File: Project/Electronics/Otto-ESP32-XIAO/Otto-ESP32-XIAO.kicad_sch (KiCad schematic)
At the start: 29 parts, among them J1 Conn_01x03, J10 Conn_01x02, J11 Conn_01x04, J12 OLED 0,91" - I2C (SKU21796), J2 Conn_01x03, J3 Conn_01x03, J4 Conn_01x03, J5 Conn_01x03, J6 Conn_01x03, J7 Conn_01x04, J8 Conn_01x06, J9 Conn_01x04, SW1 SW_SPDT, U1 MOUDLE-SEEEDUINO-XIAO-ESP32C3, U2 R-78E5.0-1.0, U3 TMC2208_SILENTSTEPSTICK, U4 TMC2208_SILENTSTEPSTICK

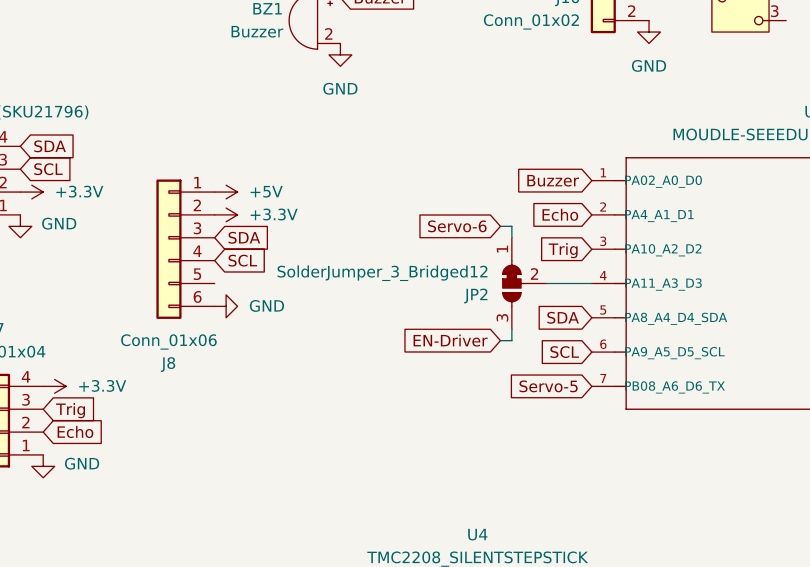
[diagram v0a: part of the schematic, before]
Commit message: quick update
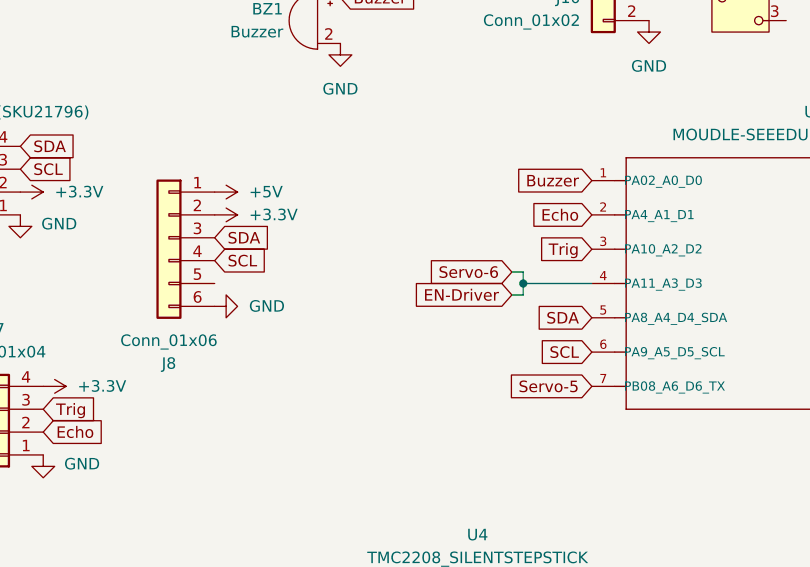
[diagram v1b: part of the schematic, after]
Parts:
- removed JP2: SolderJumper_3_Bridged12, Jumper:SolderJumper-3_P1.3mm_Bridged12_RoundedPad1.0x1.5mm, symbol Jumper:SolderJumper_3_Bridged12
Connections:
- net Servo-6 is gone; now on net EN-Driver: J6.1 (Pin_1)
- net EN-Driver: now also U1.4 (PA11_A3_D3)
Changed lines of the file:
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@@
 	)
 	(junction
+		(at 114.3 88.9)
+		(diameter 0)
+		(color 0 0 0 0)
+	)
+	(junction
 		(at 200.66 102.87)
 		(diameter 0)
@@
 	(wire
 		(pts
-			(xy 113.03 95.25) (xy 113.03 93.98)
+			(xy 213.36 102.87) (xy 200.66 102.87)
 		)
 		(stroke
@@
 	(wire
 		(pts
-			(xy 213.36 102.87) (xy 200.66 102.87)
+			(xy 213.36 111.76) (xy 200.66 111.76)
 		)
 		(stroke
@@
 	(wire
 		(pts
-			(xy 213.36 111.76) (xy 200.66 111.76)
+			(xy 114.3 88.9) (xy 121.92 88.9)
 		)
 		(stroke
@@
 	(wire
 		(pts
-			(xy 111.76 82.55) (xy 113.03 82.55)
+			(xy 194.31 144.78) (xy 191.77 144.78)
 		)
 		(stroke
@@
 	(wire
 		(pts
-			(xy 194.31 144.78) (xy 191.77 144.78)
+			(xy 114.3 87.63) (xy 114.3 88.9)
 		)
 		(stroke
@@
 	(wire
 		(pts
-			(xy 200.66 102.87) (xy 200.66 100.33)
+			(xy 113.03 90.17) (xy 114.3 90.17)
 		)
 		(stroke
@@
 	(wire
 		(pts
-			(xy 127 139.7) (xy 129.54 137.16)
+			(xy 200.66 102.87) (xy 200.66 100.33)
 		)
 		(stroke
@@
 	(wire
 		(pts
-			(xy 127 137.16) (xy 129.54 139.7)
+			(xy 113.03 87.63) (xy 114.3 87.63)
 		)
 		(stroke
@@
 	(wire
 		(pts
-			(xy 116.84 88.9) (xy 121.92 88.9)
+			(xy 127 139.7) (xy 129.54 137.16)
 		)
 		(stroke
@@
 	(wire
 		(pts
-			(xy 111.76 95.25) (xy 113.03 95.25)
+			(xy 127 137.16) (xy 129.54 139.7)
 		)
 		(stroke
@@
 	(wire
 		(pts
-			(xy 200.66 111.76) (xy 200.66 102.87)
+			(xy 114.3 88.9) (xy 114.3 90.17)
 		)
 		(stroke
@@
 	(wire
 		(pts
-			(xy 191.77 137.16) (xy 194.31 139.7)
+			(xy 200.66 111.76) (xy 200.66 102.87)
 		)
 		(stroke
@@
 	(wire
 		(pts
-			(xy 113.03 82.55) (xy 113.03 83.82)
+			(xy 191.77 137.16) (xy 194.31 139.7)
 		)
 		(stroke
@@
 	(global_label "Servo-6"
 		(shape input)
-		(at 111.76 82.55 180)
+		(at 113.03 87.63 180)
 		(fields_autoplaced yes)
 		(effects
@@
 		)
 		(property "Intersheetrefs" "${INTERSHEET_REFS}"
-			(at 100.792 82.55 0)
+			(at 102.062 87.63 0)
 			(effects
 				(font
@@
 	(global_label "EN-Driver"
 		(shape input)
-		(at 111.76 95.25 180)
+		(at 113.03 90.17 180)
 		(fields_autoplaced yes)
 		(effects
@@
 		)
 		(property "Intersheetrefs" "${INTERSHEET_REFS}"
-			(at 99.2195 95.25 0)
+			(at 100.4895 90.17 0)
 			(effects
 				(font
@@
 					(unit 1)
 				)
-			)
-		)
-	)
-	(symbol
-		(lib_id "Jumper:SolderJumper_3_Bridged12")
-		(at 113.03 88.9 90)
-		(mirror x)
-		(unit 1)
-		(exclude_from_sim yes)
-		(in_bom no)
-		(on_board yes)
-		(dnp no)
-		(property "Reference" "JP2"
-			(at 110.49 90.1701 90)
-			(effects
-				(font
-					(size 1.27 1.27)
-				)
-				(justify left)
-			)
-		)
-		(property "Value" "SolderJumper_3_Bridged12"
-			(at 110.49 87.6301 90)
-			(effects
-				(font
-					(size 1.27 1.27)
-				)
-				(justify left)
-			)
-		)
-		(property "Footprint" "Jumper:SolderJumper-3_P1.3mm_Bridged12_RoundedPad1.0x1.5mm"
-			(at 113.03 88.9 0)
-			(effects
-				(font
-					(size 1.27 1.27)
-				)
-				(hide yes)
-			)
-		)
-		(property "Datasheet" "~"
-			(at 113.03 88.9 0)
-			(effects
-				(font
-					(size 1.27 1.27)
-				)
-				(hide yes)
-			)
-		)
-		(property "Description" "3-pole Solder Jumper, pins 1+2 closed/bridged"
-			(at 113.03 88.9 0)
-			(effects
-				(font
-					(size 1.27 1.27)
-				)
-				(hide yes)
-			)
-		)
-		(pin "2"
-		)
-		(pin "1"
-		)
-		(pin "3"
-		)
-		(instances
-			(project ""
-				(path "/d2682c99-4285-4c0b-9e61-08b763b3ce0d"
-					(reference "JP2")
-					(unit 1)
-				)
